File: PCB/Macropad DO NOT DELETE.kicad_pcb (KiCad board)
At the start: 2 copper layers, 64 x 61 mm, 9 parts, among them SW1 SW_Push, SW10 RotaryEncoder, SW2 SW_Push, SW3 SW_Push, SW4 SW_Push, SW5 SW_Push, SW9 RotaryEncoder, U1 MOUDLE-SEEEDUINO-XIAO, U2 ER_OLEDM0.91_1x-I2C

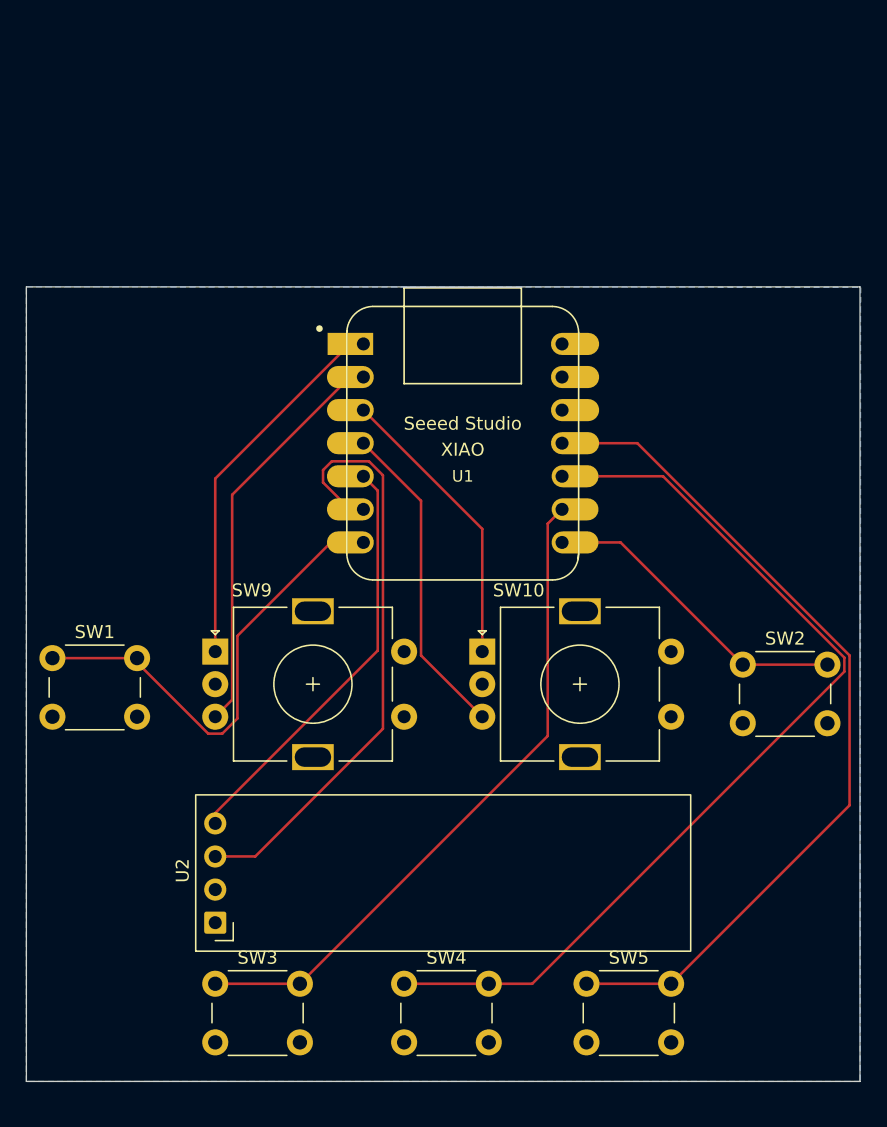
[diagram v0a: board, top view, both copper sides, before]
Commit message: after rechecking
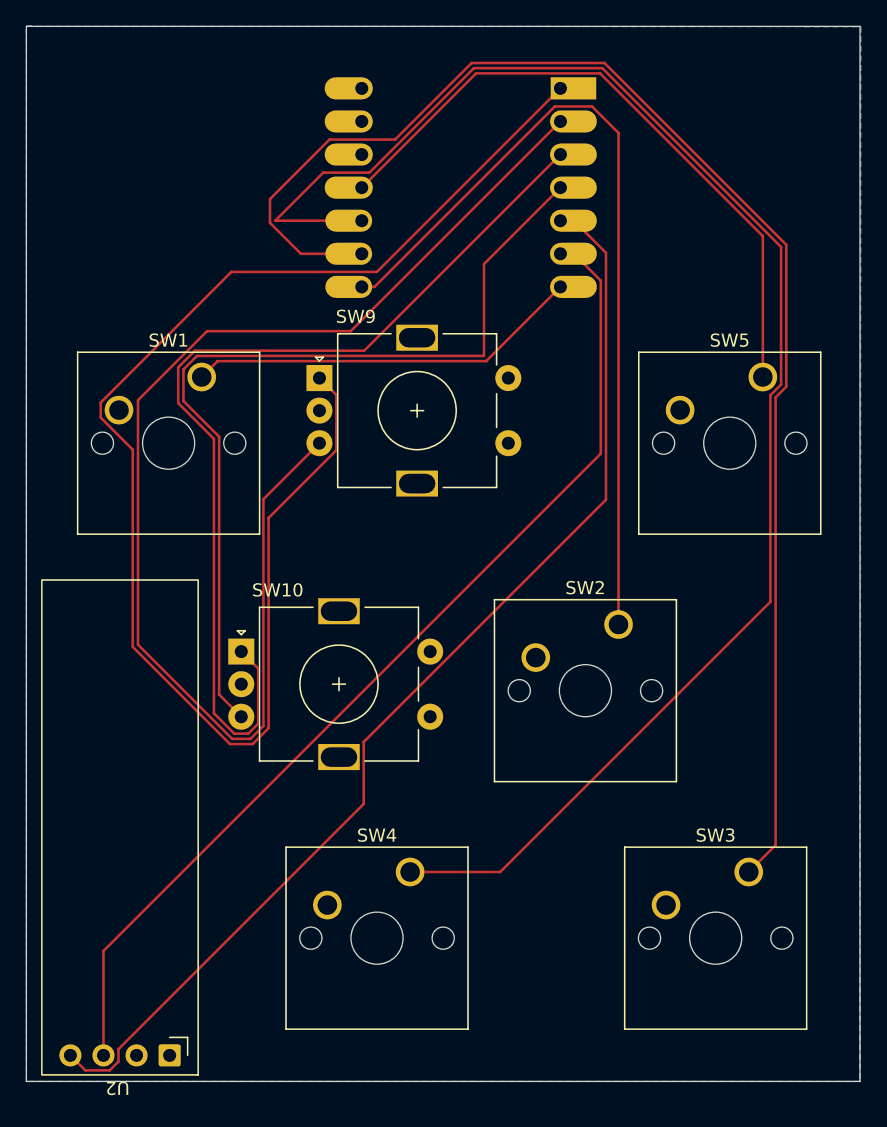
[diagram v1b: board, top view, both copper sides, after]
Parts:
- SW1, SW2, SW3, SW4, SW5: footprint Button_Switch_THT:SW_PUSH_6mm -> Button_Switch_Keyboard:SW_Cherry_MX_1.00u_PCB
- U1: moved to B.Cu
- moved SW5 48.5 mm to (179.5, 74.9)
- moved SW3 41.8 mm to (178.5, 112.9)
- moved SW1 24.4 mm to (136.5, 74.9)
- moved SW9 22.5 mm to (145.5, 75.0)
- moved U1 19.6 mm to (156.4, 60.4), turned to 180 degrees
- moved SW10 18.5 mm to (139.5, 96.0)
- moved U2 10.8 mm to (134.0, 127.0), turned to 180 degrees
- moved SW2 10.0 mm to (168.5, 93.9)
- moved SW4 8.59 mm to (152.5, 112.9)
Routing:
- net Net-(U1-PA02_A0_D0): track 28.9 -> 108.7 mm
- net Net-(U1-PA4_A1_D1): track 31.4 -> 96.6 mm
- net Net-(U1-PA7_A8_D8_SCK): track 51.3 -> 108.9 mm
- net Net-(U1-PA8_A4_D4_SDA): track 32.3 -> 86.6 mm
- net Net-(U1-PA10_A2_D2): track 22.3 -> 74.2 mm
- net Net-(U1-PA5_A9_D9_MISO): track 72.2 -> 119.9 mm
- net Net-(U1-PA11_A3_D3): track 24.8 -> 67.4 mm
- net Net-(U1-PB09_A7_D7_RX): track 24.3 -> 64.0 mm
- net Net-(U1-PA9_A5_D5_SCL): track 46.6 -> 79.2 mm
- net Net-(U1-PA6_A10_D10_MOSI): track 66.2 -> 50.4 mm
- net Net-(U1-PB08_A6_D6_TX): track 36.3 -> 30.4 mm
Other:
- board size 64 x 61 mm -> 64 x 81 mm
